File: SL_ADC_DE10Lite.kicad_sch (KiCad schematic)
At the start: 23 parts, among them J1 DE10Lite header, J2 Analog header

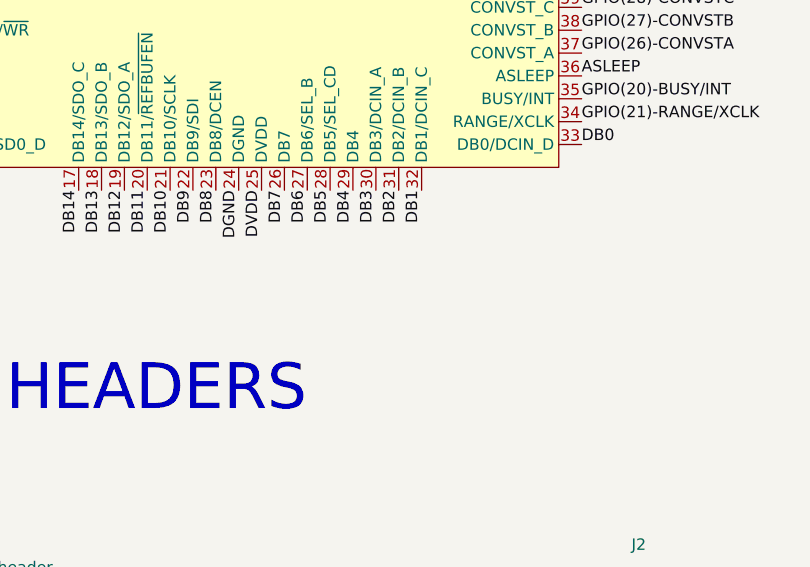
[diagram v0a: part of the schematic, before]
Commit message: updated?
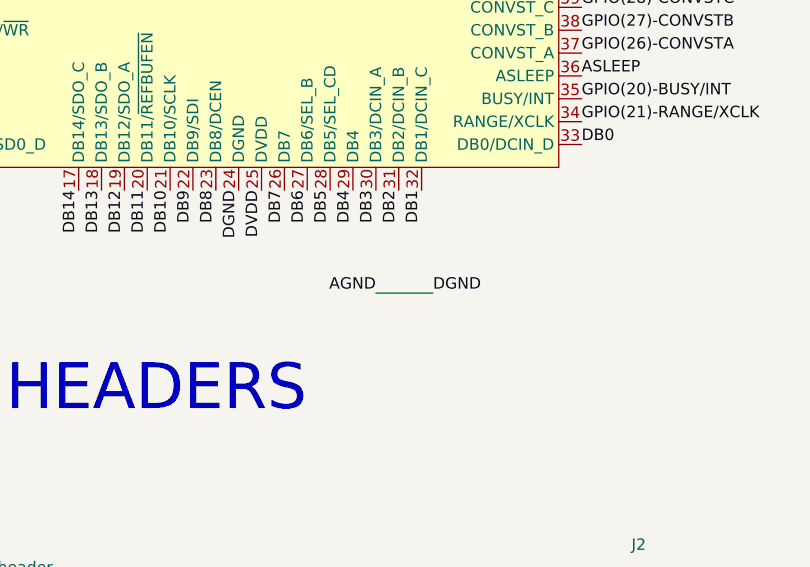
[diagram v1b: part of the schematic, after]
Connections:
- net DGND is gone; now on net AGND: C5.2, IC1.24 (DGND), J1.12 (Pin_12), J1.30 (Pin_30), J2.27 (Pin_27), J2.28 (Pin_28)
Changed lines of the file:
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@@
+	(wire
+		(pts
+			(xy 93.98 96.52) (xy 100.33 96.52)
+		)
+		(stroke
+			(width 0)
+			(type default)
+		)
+	)
 	(wire
 		(pts
@@
 		)
 	)
+	(label "AGND"
+		(at 93.98 96.52 180)
+		(effects
+			(font
+				(size 1.27 1.27)
+			)
+			(justify right bottom)
+		)
+	)
 	(label "AVDD"
 		(at 43.18 74.93 180)
@@
 		)
 	)
+	(label "DGND"
+		(at 100.33 96.52 0)
+		(effects
+			(font
+				(size 1.27 1.27)
+			)
+			(justify left bottom)
+		)
+	)
